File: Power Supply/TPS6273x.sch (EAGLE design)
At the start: 5 parts

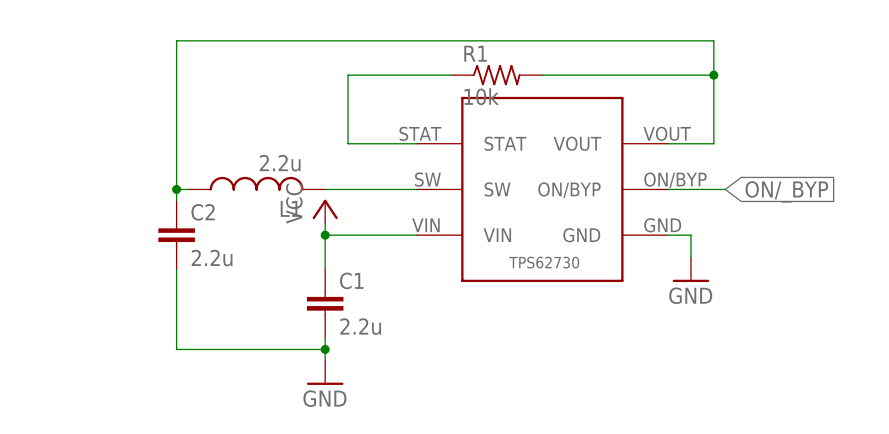
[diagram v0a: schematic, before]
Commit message: mq updated
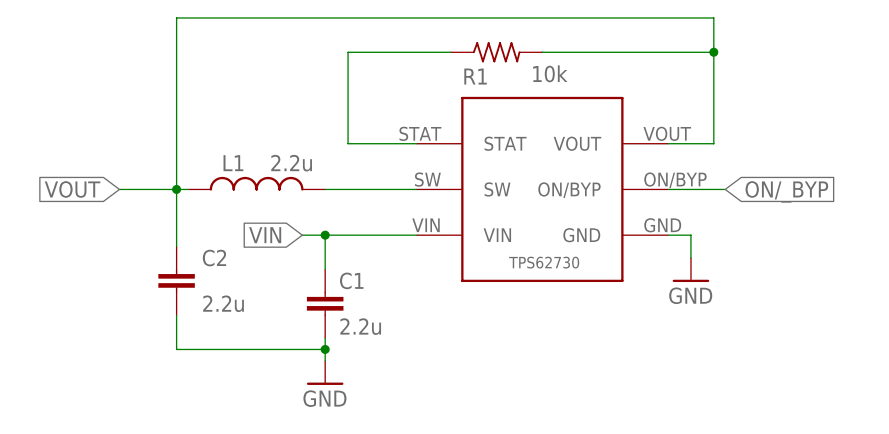
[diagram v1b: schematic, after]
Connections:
- net N$3 renamed VOUT
- net VCC renamed VIN
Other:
- moved on the sheet: C2, R1
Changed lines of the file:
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@@
 <?xml version="1.0" encoding="utf-8"?>
 <!DOCTYPE eagle SYSTEM "eagle.dtd">
-<eagle version="9.6.2">
+<eagle version="7.5.0">
 <drawing>
 <settings>
@@
 <part name="U$1" library="TI-TPS6273X" deviceset="TPS62730" device=""/>
 <part name="L1" library="rcl-2" deviceset="L-US" device="L1210" value="2.2u"/>
-<part name="C1" library="rcl" library_urn="urn:adsk.eagle:library:334" deviceset="C-EU" device="C0603" package3d_urn="urn:adsk.eagle:package:23616/2" value="2.2u"/>
-<part name="C2" library="rcl" library_urn="urn:adsk.eagle:library:334" deviceset="C-EU" device="C0603" package3d_urn="urn:adsk.eagle:package:23616/2" value="2.2u"/>
-<part name="P+1" library="supply1" library_urn="urn:adsk.eagle:library:371" deviceset="VCC" device=""/>
-<part name="GND1" library="supply1" library_urn="urn:adsk.eagle:library:371" deviceset="GND" device=""/>
-<part name="GND2" library="supply1" library_urn="urn:adsk.eagle:library:371" deviceset="GND" device=""/>
-<part name="R1" library="rcl" library_urn="urn:adsk.eagle:library:334" deviceset="R-US_" device="R0603" package3d_urn="urn:adsk.eagle:package:23555/3" value="10k"/>
+<part name="C1" library="rcl" deviceset="C-EU" device="C0603" value="2.2u"/>
+<part name="C2" library="rcl" deviceset="C-EU" device="C0603" value="2.2u"/>
+<part name="GND1" library="supply1" deviceset="GND" device=""/>
+<part name="GND2" library="supply1" deviceset="GND" device=""/>
+<part name="R1" library="rcl" deviceset="R-US_" device="R0603" value="10k"/>
 </parts>
 <sheets>
@@
 <instance part="U$1" gate="G$1" x="50.8" y="58.42" smashed="yes"/>
 <instance part="L1" gate="G$1" x="25.4" y="66.04" smashed="yes" rot="R90">
-<attribute name="NAME" x="30.48" y="64.77" size="1.778" layer="95" rot="R180"/>
-<attribute name="VALUE" x="30.48" y="69.85" size="1.778" layer="96" rot="R180"/>
+<attribute name="NAME" x="24.13" y="69.85" size="1.778" layer="95" rot="R180"/>
+<attribute name="VALUE" x="31.75" y="69.85" size="1.778" layer="96" rot="R180"/>
 </instance>
 <instance part="C1" gate="G$1" x="33.02" y="54.61" smashed="yes">
@@
 <attribute name="VALUE" x="34.544" y="49.911" size="1.778" layer="96"/>
 </instance>
-<instance part="C2" gate="G$1" x="16.51" y="62.23" smashed="yes">
-<attribute name="NAME" x="18.034" y="62.611" size="1.778" layer="95"/>
-<attribute name="VALUE" x="18.034" y="57.531" size="1.778" layer="96"/>
-</instance>
-<instance part="P+1" gate="VCC" x="33.02" y="64.77" smashed="yes">
-<attribute name="VALUE" x="30.48" y="62.23" size="1.778" layer="96" rot="R90"/>
+<instance part="C2" gate="G$1" x="16.51" y="57.15" smashed="yes">
+<attribute name="NAME" x="19.304" y="57.531" size="1.778" layer="95"/>
+<attribute name="VALUE" x="19.304" y="52.451" size="1.778" layer="96"/>
 </instance>
 <instance part="GND1" gate="1" x="33.02" y="44.45" smashed="yes">
@@
 <attribute name="VALUE" x="71.12" y="53.34" size="1.778" layer="96"/>
 </instance>
-<instance part="R1" gate="G$1" x="52.07" y="78.74" smashed="yes">
-<attribute name="NAME" x="48.26" y="80.2386" size="1.778" layer="95"/>
-<attribute name="VALUE" x="48.26" y="75.438" size="1.778" layer="96"/>
+<instance part="R1" gate="G$1" x="52.07" y="81.28" smashed="yes">
+<attribute name="NAME" x="48.26" y="77.6986" size="1.778" layer="95"/>
+<attribute name="VALUE" x="55.88" y="77.978" size="1.778" layer="96"/>
 </instance>
 </instances>
@@
 <pinref part="C2" gate="G$1" pin="2"/>
 <wire x1="33.02" y1="48.26" x2="33.02" y2="49.53" width="0.1524" layer="91"/>
-<wire x1="16.51" y1="57.15" x2="16.51" y2="48.26" width="0.1524" layer="91"/>
+<wire x1="16.51" y1="52.07" x2="16.51" y2="48.26" width="0.1524" layer="91"/>
 <wire x1="16.51" y1="48.26" x2="33.02" y2="48.26" width="0.1524" layer="91"/>
 <junction x="33.02" y="48.26"/>
@@
 </segment>
 </net>
-<net name="VCC" class="0">
+<net name="N$2" class="0">
+<segment>
+<pinref part="U$1" gate="G$1" pin="SW"/>
+<pinref part="L1" gate="G$1" pin="2"/>
+<wire x1="43.18" y1="66.04" x2="33.02" y2="66.04" width="0.1524" layer="91"/>
+</segment>
+</net>
+<net name="N$5" class="0">
+<segment>
+<pinref part="U$1" gate="G$1" pin="STAT"/>
+<wire x1="43.18" y1="71.12" x2="35.56" y2="71.12" width="0.1524" layer="91"/>
+<wire x1="35.56" y1="71.12" x2="35.56" y2="81.28" width="0.1524" layer="91"/>
+<pinref part="R1" gate="G$1" pin="1"/>
+<wire x1="35.56" y1="81.28" x2="46.99" y2="81.28" width="0.1524" layer="91"/>
+</segment>
+</net>
+<net name="ON/_BYP" class="0">
+<segment>
+<pinref part="U$1" gate="G$1" pin="ON/BYP"/>
+<wire x1="71.12" y1="66.04" x2="77.47" y2="66.04" width="0.1524" layer="91"/>
+<label x="77.47" y="66.04" size="1.778" layer="95" xref="yes"/>
+</segment>
+</net>
+<net name="VIN" class="0">
 <segment>
 <pinref part="C1" gate="G$1" pin="1"/>
@@
 <pinref part="U$1" gate="G$1" pin="VIN"/>
 <wire x1="33.02" y1="60.96" x2="43.18" y2="60.96" width="0.1524" layer="91"/>
-<pinref part="P+1" gate="VCC" pin="VCC"/>
-<wire x1="33.02" y1="62.23" x2="33.02" y2="60.96" width="0.1524" layer="91"/>
+<label x="30.48" y="60.96" size="1.778" layer="95" rot="R180" xref="yes"/>
+<wire x1="33.02" y1="60.96" x2="30.48" y2="60.96" width="0.1524" layer="91"/>
 <junction x="33.02" y="60.96"/>
 </segment>
 </net>
-<net name="N$2" class="0">
-<segment>
-<pinref part="U$1" gate="G$1" pin="SW"/>
-<pinref part="L1" gate="G$1" pin="2"/>
-<wire x1="43.18" y1="66.04" x2="33.02" y2="66.04" width="0.1524" layer="91"/>
-</segment>
-</net>
-<net name="N$3" class="0">
-<segment>
+<net name="VOUT" class="0">
+<segment>
+<wire x1="10.16" y1="66.04" x2="16.51" y2="66.04" width="0.1524" layer="91"/>
 <pinref part="L1" gate="G$1" pin="1"/>
 <wire x1="17.78" y1="66.04" x2="16.51" y2="66.04" width="0.1524" layer="91"/>
 <pinref part="C2" gate="G$1" pin="1"/>
-<wire x1="16.51" y1="66.04" x2="16.51" y2="64.77" width="0.1524" layer="91"/>
+<wire x1="16.51" y1="66.04" x2="16.51" y2="59.69" width="0.1524" layer="91"/>
 <pinref part="U$1" gate="G$1" pin="VOUT"/>
 <wire x1="71.12" y1="71.12" x2="76.2" y2="71.12" width="0.1524" layer="91"/>
-<wire x1="76.2" y1="71.12" x2="76.2" y2="78.74" width="0.1524" layer="91"/>
-<wire x1="76.2" y1="78.74" x2="76.2" y2="82.55" width="0.1524" layer="91"/>
-<wire x1="76.2" y1="82.55" x2="16.51" y2="82.55" width="0.1524" layer="91"/>
-<wire x1="16.51" y1="82.55" x2="16.51" y2="66.04" width="0.1524" layer="91"/>
+<wire x1="76.2" y1="71.12" x2="76.2" y2="81.28" width="0.1524" layer="91"/>
+<wire x1="76.2" y1="81.28" x2="76.2" y2="85.09" width="0.1524" layer="91"/>
+<wire x1="76.2" y1="85.09" x2="16.51" y2="85.09" width="0.1524" layer="91"/>
+<wire x1="16.51" y1="85.09" x2="16.51" y2="66.04" width="0.1524" layer="91"/>
 <junction x="16.51" y="66.04"/>
 <pinref part="R1" gate="G$1" pin="2"/>
-<wire x1="57.15" y1="78.74" x2="76.2" y2="78.74" width="0.1524" layer="91"/>
-<junction x="76.2" y="78.74"/>
-</segment>
-</net>
-<net name="N$5" class="0">
-<segment>
-<pinref part="U$1" gate="G$1" pin="STAT"/>
-<wire x1="43.18" y1="71.12" x2="35.56" y2="71.12" width="0.1524" layer="91"/>
-<wire x1="35.56" y1="71.12" x2="35.56" y2="78.74" width="0.1524" layer="91"/>
-<pinref part="R1" gate="G$1" pin="1"/>
-<wire x1="35.56" y1="78.74" x2="46.99" y2="78.74" width="0.1524" layer="91"/>
-</segment>
-</net>
-<net name="ON/_BYP" class="0">
-<segment>
-<pinref part="U$1" gate="G$1" pin="ON/BYP"/>
-<wire x1="71.12" y1="66.04" x2="77.47" y2="66.04" width="0.1524" layer="91"/>
-<label x="77.47" y="66.04" size="1.778" layer="95" xref="yes"/>
+<wire x1="57.15" y1="81.28" x2="76.2" y2="81.28" width="0.1524" layer="91"/>
+<junction x="76.2" y="81.28"/>
+<label x="10.16" y="66.04" size="1.778" layer="95" rot="R180" xref="yes"/>
 </segment>
 </net>
@@
 </schematic>
 </drawing>
-<compatibility>
-<note version="8.2" severity="warning">
-Since Version 8.2, EAGLE supports online libraries. The ids
-of those online libraries will not be understood (or retained)
-with this version.
-</note>
-<note version="8.3" severity="warning">
-Since Version 8.3, EAGLE supports URNs for individual library
-assets (packages, symbols, and devices). The URNs of those assets
-will not be understood (or retained) with this version.
-</note>
-<note version="8.3" severity="warning">
-Since Version 8.3, EAGLE supports the association of 3D packages
-with devices in libraries, schematics, and board files. Those 3D
-packages will not be understood (or retained) with this version.
-</note>
-<note version="8.4" severity="warning">
-Since Version 8.4, EAGLE supports properties for SPICE simulation.
-Probes in schematics and SPICE mapping objects found in parts and library devices
-will not be understood with this version. Update EAGLE to the latest version
-for full support of SPICE simulation.
-</note>
-</compatibility>
 </eagle>
